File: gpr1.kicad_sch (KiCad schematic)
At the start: 10 parts, among them U16 74HCT541, U17 74HCT00, U18 74HCT04, U4 74HCT138, U7 74HCT574

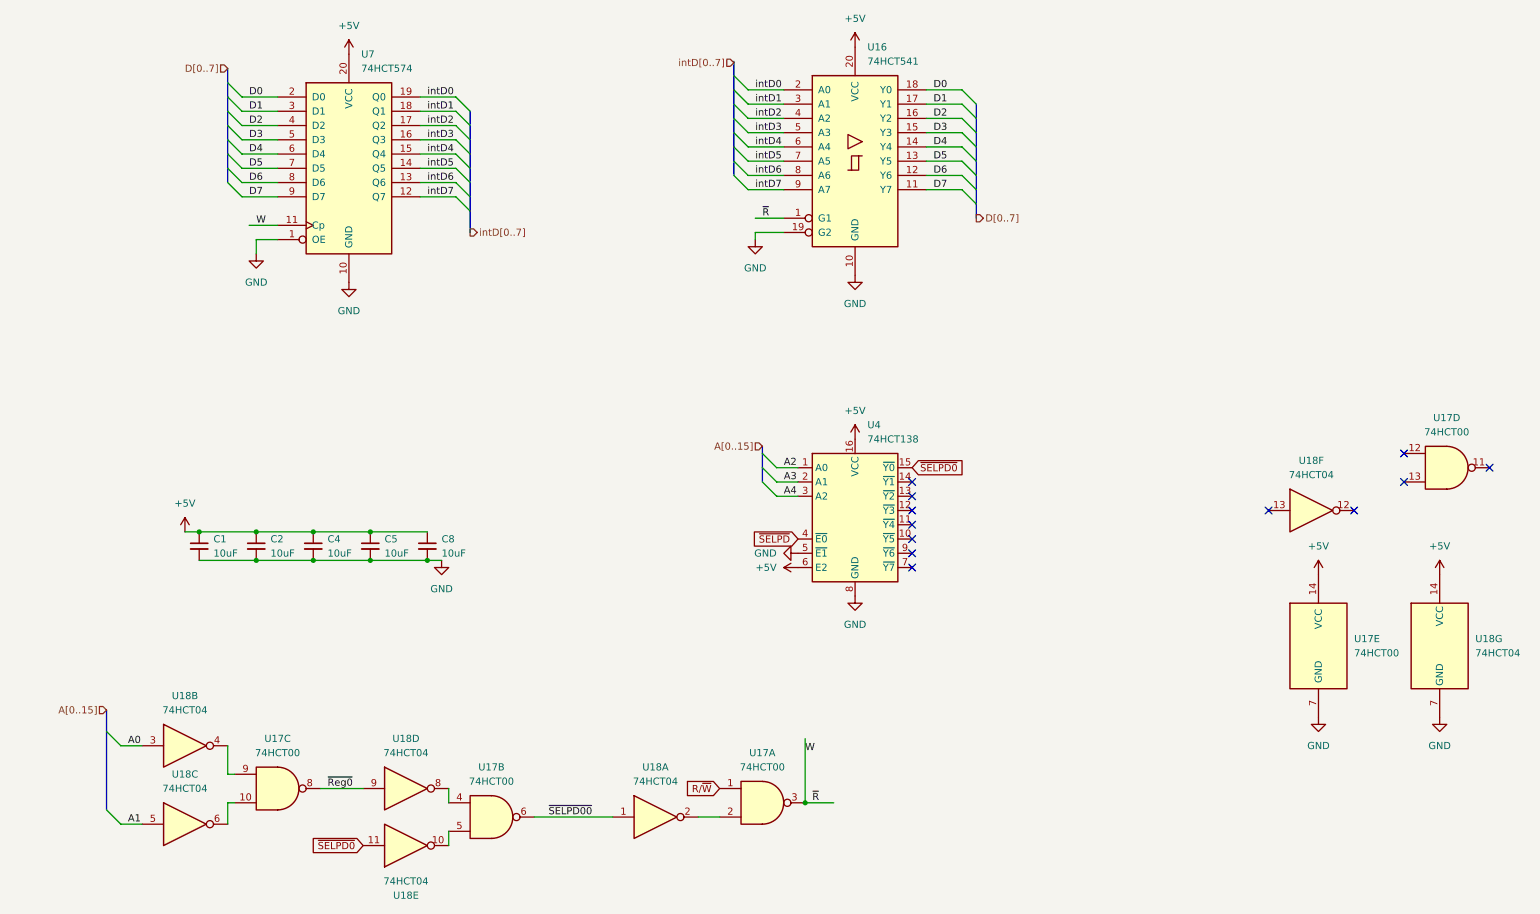
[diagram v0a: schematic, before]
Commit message: tighten up tracing
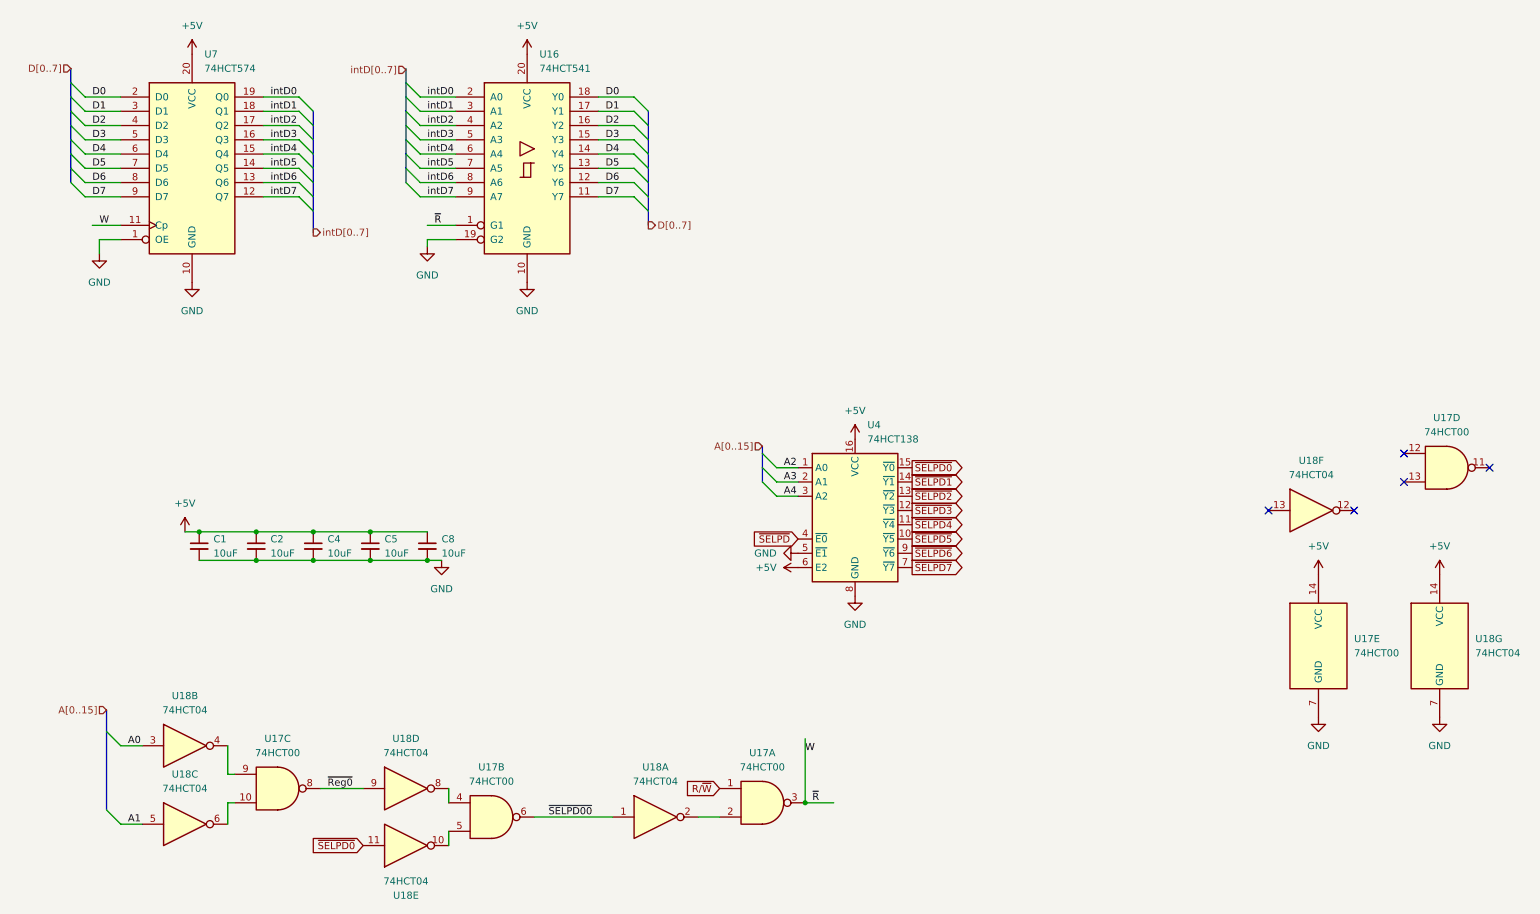
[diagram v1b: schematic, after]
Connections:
- net ~{SELPD5}: now reaches U4.10 (~{Y5})
- net ~{SELPD4}: now reaches U4.11 (~{Y4})
- net ~{SELPD3}: now reaches U4.12 (~{Y3})
- net ~{SELPD2}: now reaches U4.13 (~{Y2})
- net ~{SELPD1}: now reaches U4.14 (~{Y1})
- net ~{SELPD7}: now reaches U4.7 (~{Y7})
- net ~{SELPD6}: now reaches U4.9 (~{Y6})
- no-connect marks 12 -> 5
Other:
- moved on the sheet: U16, U7

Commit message: clean up before redesign
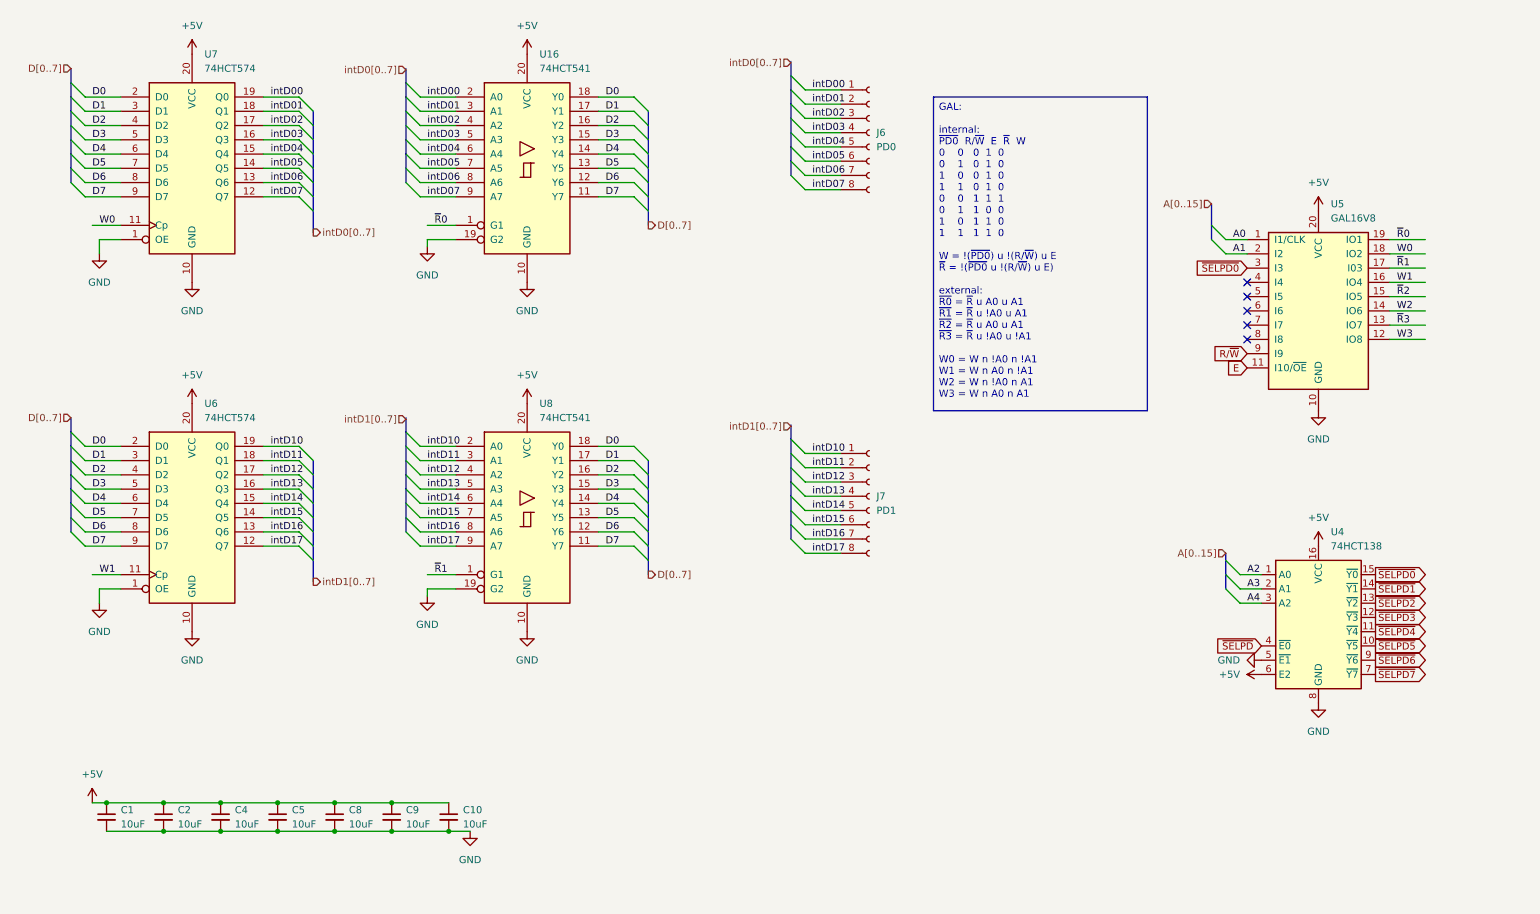
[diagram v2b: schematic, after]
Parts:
- removed U17: 74HCT00, Package_SO:SOIC-14_3.9x8.7mm_P1.27mm, symbol 74xx:74HCT00
- removed U18: 74HCT04, Package_SO:SOIC-14_3.9x8.7mm_P1.27mm, symbol 74xx:74HCT04
- added C10, C9: 10uF, Capacitor_SMD:C_0805_2012Metric_Pad1.18x1.45mm_HandSolder, symbol Device:C_Small
- added J6: PD0, Connector_PinSocket_2.54mm:PinSocket_1x08_P2.54mm_Vertical, symbol Connector:Conn_01x08_Socket
- added J7: PD1, Connector_PinSocket_2.54mm:PinSocket_1x08_P2.54mm_Vertical, symbol Connector:Conn_01x08_Socket
- added U5: GAL16V8, Package_DIP:DIP-20_W7.62mm, symbol Logic_Programmable:GAL16V8
- added U6: 74HCT574, Package_SO:SOIC-20W_7.5x12.8mm_P1.27mm, symbol 74xx:74LS574
- added U8: 74HCT541, Package_SO:SOIC-20W_7.5x12.8mm_P1.27mm, symbol 74xx:74LS541
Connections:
- net +5V: now also C10.1, C9.1, U5.20 (VCC), U6.20 (VCC), U8.20 (VCC)
- net A0: now also U5.1 (I1/CLK)
- net A1: now also U5.2 (I2)
- net D0: now also U6.2 (D0), U8.18 (Y0)
- net D1: now also U6.3 (D1), U8.17 (Y1)
- net D2: now also U6.4 (D2), U8.16 (Y2)
- net D3: now also U6.5 (D3), U8.15 (Y3)
- net D4: now also U6.6 (D4), U8.14 (Y4)
- net D5: now also U6.7 (D5), U8.13 (Y5)
- net D6: now also U6.8 (D6), U8.12 (Y6)
- net D7: now also U6.9 (D7), U8.11 (Y7)
- net GND: now also C10.2, C9.2, U5.10 (GND), U6.1 (OE), U6.10 (GND), U8.10 (GND), U8.19 (G2)
- net R/~{W}: now also U5.9 (I9)
- net ~{SELPD0}: now also U5.3 (I3)
- net W renamed W0
- net W0: now also U5.18 (IO2); no longer U16.1 (G1)
- net intD0 renamed intD00
- net intD00: now also J6.1 (Pin_1)
- net intD1 renamed intD01
- net intD01: now also J6.2 (Pin_2)
- net intD2 renamed intD02
- net intD02: now also J6.3 (Pin_3)
- net intD3 renamed intD03
- net intD03: now also J6.4 (Pin_4)
- net intD4 renamed intD04
- net intD04: now also J6.5 (Pin_5)
- net intD5 renamed intD05
- net intD05: now also J6.6 (Pin_6)
- net intD6 renamed intD06
- net intD06: now also J6.7 (Pin_7)
- net intD7 renamed intD07
- net intD07: now also J6.8 (Pin_8)
- new net E: U5.11 (I10/~{OE})
- new net W1: U5.16 (IO4), U6.11 (Cp)
- new net W2: U5.14 (IO6)
- new net W3: U5.12 (IO8)
- new net intD10: J7.1 (Pin_1), U6.19 (Q0), U8.2 (A0)
- new net intD11: J7.2 (Pin_2), U6.18 (Q1), U8.3 (A1)
- new net intD12: J7.3 (Pin_3), U6.17 (Q2), U8.4 (A2)
- new net intD13: J7.4 (Pin_4), U6.16 (Q3), U8.5 (A3)
- new net intD14: J7.5 (Pin_5), U6.15 (Q4), U8.6 (A4)
- new net intD15: J7.6 (Pin_6), U6.14 (Q5), U8.7 (A5)
- new net intD16: J7.7 (Pin_7), U6.13 (Q6), U8.8 (A6)
- new net intD17: J7.8 (Pin_8), U6.12 (Q7), U8.9 (A7)
- new net ~{R}0: U16.1 (G1), U5.19 (IO1)
- new net ~{R}1: U5.17 (I03), U8.1 (G1)
- new net ~{R}2: U5.15 (IO5)
- new net ~{R}3: U5.13 (IO7)
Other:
- moved on the sheet: C1, C2, C4, C5, C8, U4
